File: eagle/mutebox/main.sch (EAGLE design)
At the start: 44 parts, among them IC1 6N138S-TA1, IC2 6N138S-TA1, IC3 74HCT541DW, IC4 74HCT541DW, IC5 74HC595D, Q1 BC337

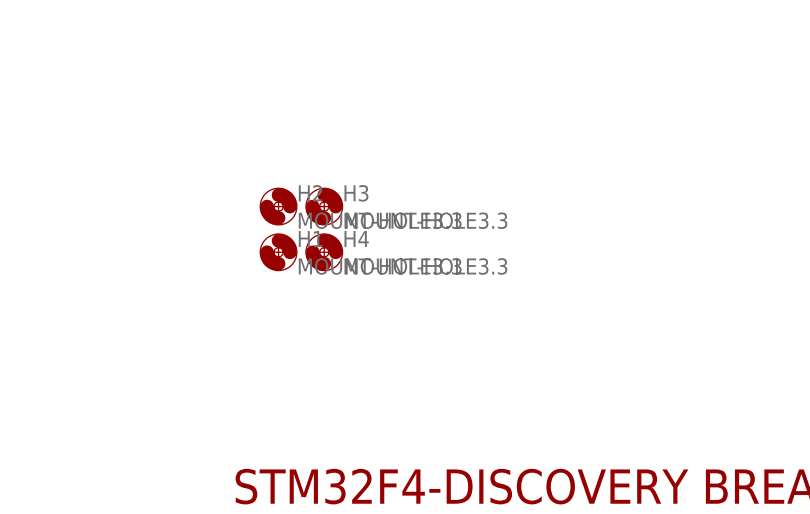
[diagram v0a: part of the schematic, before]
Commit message: wip
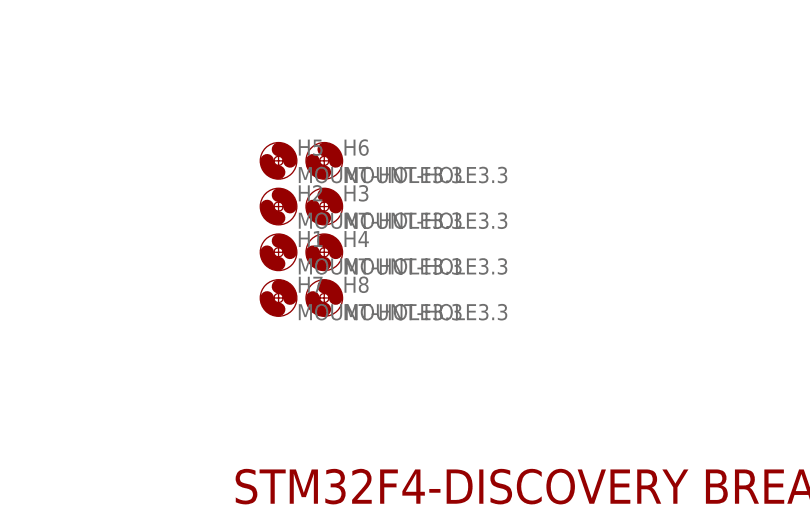
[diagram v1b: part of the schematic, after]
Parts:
- added H5, H6, H7, H8: MOUNT-HOLE3.3, holes:MOUNT-HOLE3.3
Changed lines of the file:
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@@
 <part name="R15" library="microbuilder" deviceset="RESISTOR" device="_0603" value="1K"/>
 <part name="CONN_LCD" library="con-harting-ml" deviceset="ML16" device=""/>
+<part name="H5" library="holes" deviceset="MOUNT-HOLE" device="3.3"/>
+<part name="H6" library="holes" deviceset="MOUNT-HOLE" device="3.3"/>
+<part name="H7" library="holes" deviceset="MOUNT-HOLE" device="3.3"/>
+<part name="H8" library="holes" deviceset="MOUNT-HOLE" device="3.3"/>
 </parts>
 <sheets>
@@
 <instance part="R15" gate="G$1" x="264.16" y="-53.34" rot="R90"/>
 <instance part="CONN_LCD" gate="1" x="342.9" y="5.08"/>
+<instance part="H5" gate="G$1" x="99.06" y="137.16"/>
+<instance part="H6" gate="G$1" x="104.14" y="137.16"/>
+<instance part="H7" gate="G$1" x="99.06" y="121.92"/>
+<instance part="H8" gate="G$1" x="104.14" y="121.92"/>
 </instances>
 <busses>
